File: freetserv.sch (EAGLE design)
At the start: 62 parts, among them IC2 SN75240PW, Q1 12MHz, Q2 6MHz, U1 MCP16311-E/MS, U4 TLV810SDBZT, U5 SN74LVC1G86DCKR

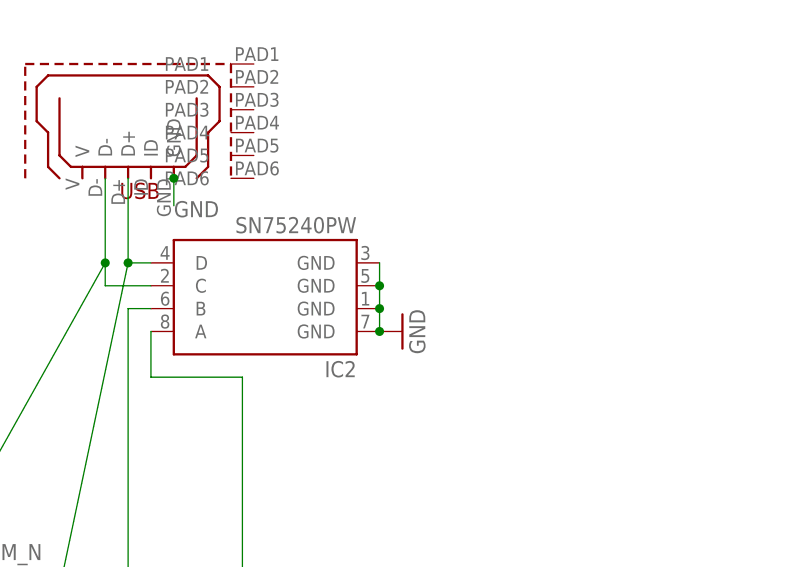
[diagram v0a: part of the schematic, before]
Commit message: address all DRC warnings
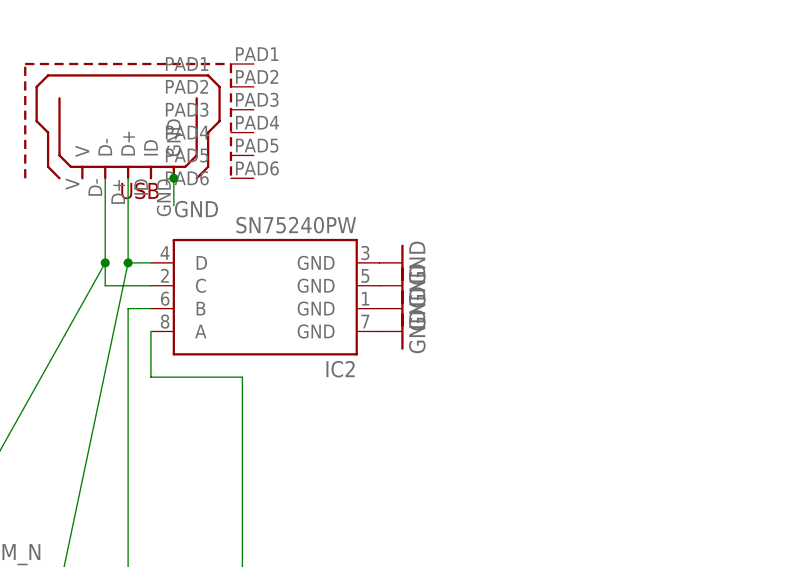
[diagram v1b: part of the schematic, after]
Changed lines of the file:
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@@
 <clearance class="1" value="0.2"/>
 </class>
-<class number="2" name="power" width="1.143" drill="0">
+<class number="2" name="power" width="0.4064" drill="0">
 </class>
 </classes>
@@
 <part name="C36" library="resistor" deviceset="C-EU" device="C0805" value="0.1uF"/>
 <part name="GND42" library="supply1" deviceset="GND" device=""/>
+<part name="GND43" library="supply1" deviceset="GND" device=""/>
+<part name="GND48" library="supply1" deviceset="GND" device=""/>
+<part name="GND49" library="supply1" deviceset="GND" device=""/>
 </parts>
 <sheets>
@@
 <instance part="C36" gate="G$1" x="-2.54" y="228.6"/>
 <instance part="GND42" gate="1" x="-2.54" y="233.68" rot="R180"/>
+<instance part="GND43" gate="1" x="119.38" y="248.92" rot="R90"/>
+<instance part="GND48" gate="1" x="119.38" y="246.38" rot="R90"/>
+<instance part="GND49" gate="1" x="119.38" y="243.84" rot="R90"/>
 </instances>
 <busses>
@@
 <pinref part="IC2" gate="G$1" pin="GND@1"/>
 <pinref part="GND8" gate="1" pin="GND"/>
-<pinref part="IC2" gate="G$1" pin="GND@4"/>
-<wire x1="116.84" y1="248.92" x2="116.84" y2="246.38" width="0.1524" layer="91"/>
-<pinref part="IC2" gate="G$1" pin="GND@2"/>
-<junction x="116.84" y="243.84"/>
-<wire x1="116.84" y1="246.38" x2="116.84" y2="243.84" width="0.1524" layer="91"/>
-<wire x1="116.84" y1="243.84" x2="116.84" y2="241.3" width="0.1524" layer="91"/>
-<pinref part="IC2" gate="G$1" pin="GND@3"/>
-<junction x="116.84" y="246.38"/>
-<junction x="116.84" y="241.3"/>
 </segment>
 <segment>
@@
 <pinref part="GND42" gate="1" pin="GND"/>
 </segment>
+<segment>
+<pinref part="IC2" gate="G$1" pin="GND@4"/>
+<pinref part="GND43" gate="1" pin="GND"/>
+</segment>
+<segment>
+<pinref part="IC2" gate="G$1" pin="GND@3"/>
+<pinref part="GND48" gate="1" pin="GND"/>
+</segment>
+<segment>
+<pinref part="IC2" gate="G$1" pin="GND@2"/>
+<pinref part="GND49" gate="1" pin="GND"/>
+</segment>
 </net>
